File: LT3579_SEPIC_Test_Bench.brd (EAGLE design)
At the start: 74 x 58 mm, 160 parts

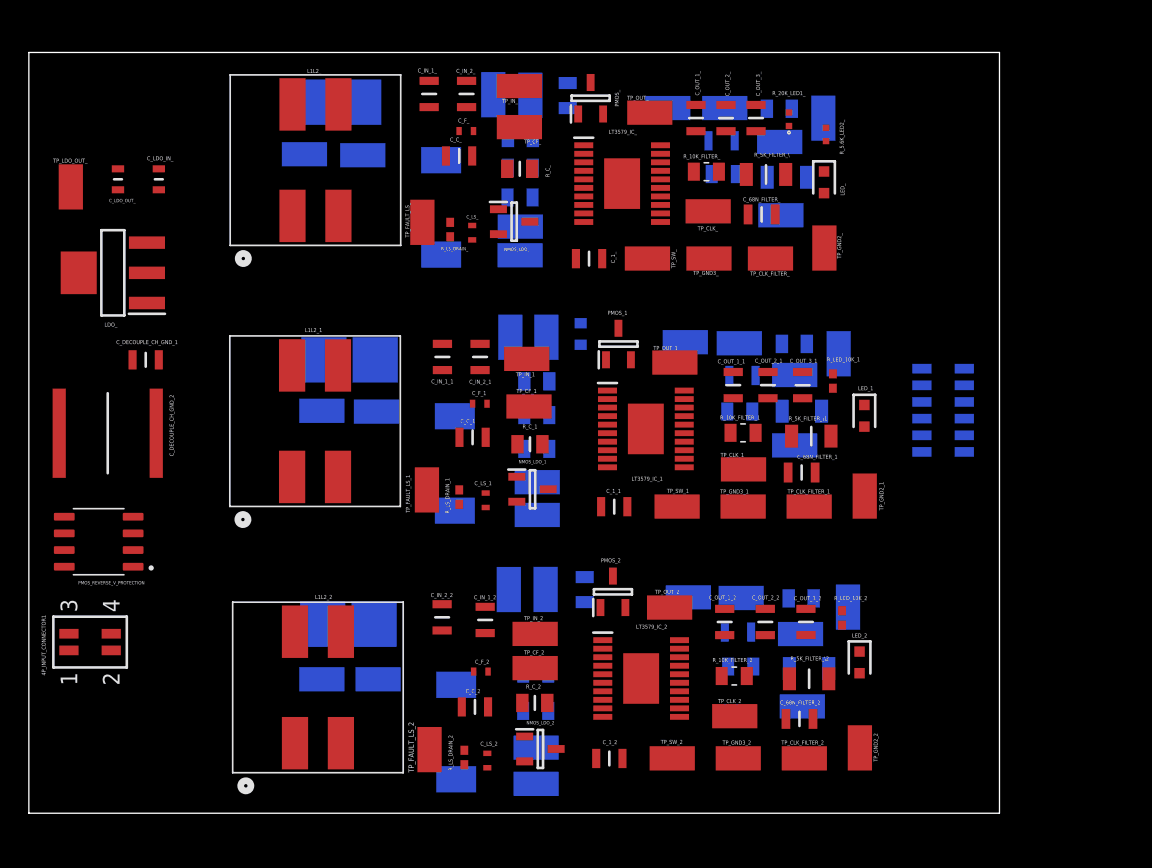
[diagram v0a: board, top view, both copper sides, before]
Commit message: modiefied baord layout
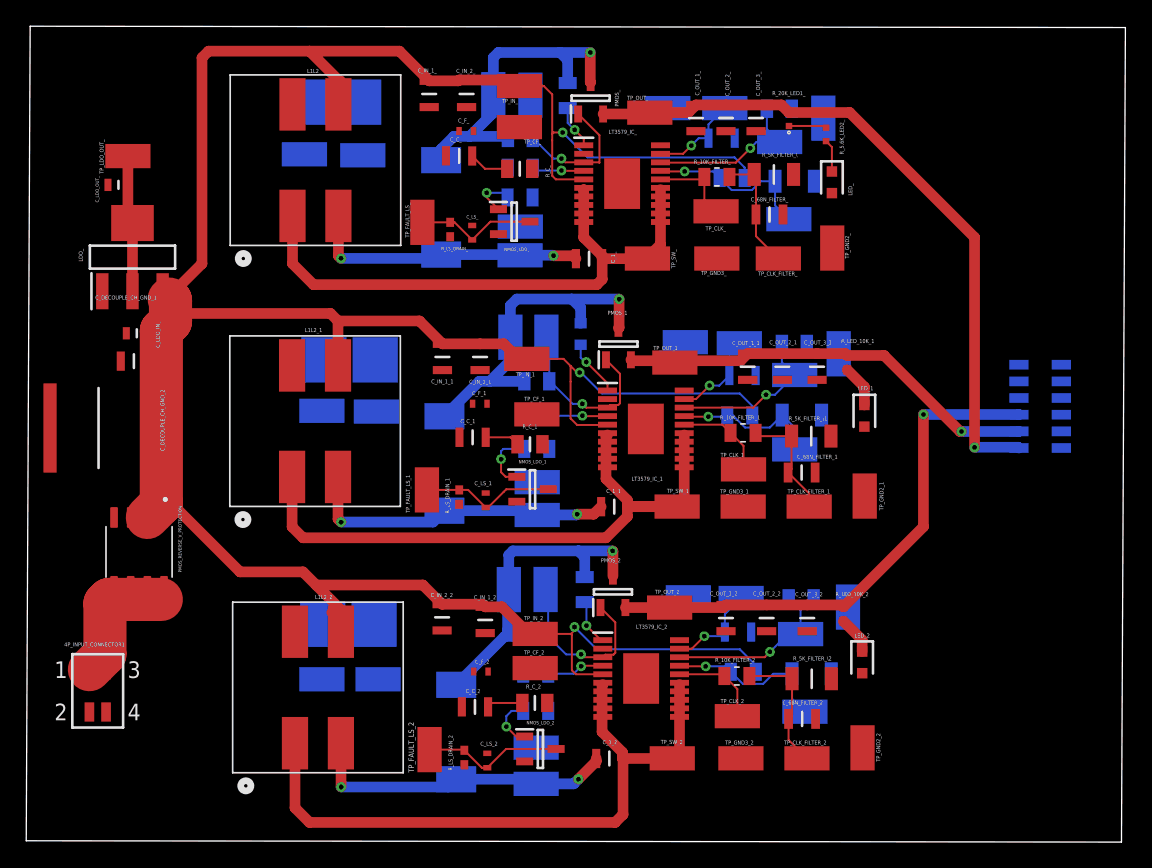
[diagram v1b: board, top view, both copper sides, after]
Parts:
- moved C_LDO_IN_ 11.9 mm to (8.23, 36.6), turned to 180 degrees
- moved 12P_OUTPUT_CONNECTOR1 7.41 mm to (77.1, 31.0)
- moved TP_LDO_OUT_ 4.94 mm to (7.55, 50.1), turned to 180 degrees
- moved 4P_INPUT_CONNECTOR1 3.76 mm to (5.25, 9.33), turned to 0 degrees
- moved PMOS_REVERSE_V_PROTECTION 3.17 mm to (8.40, 19.9), turned to 270 degrees
- moved LDO_ 1.92 mm to (7.90, 42.4), turned to 90 degrees
- moved C_OUT_2_1 1.78 mm to (57.4, 34.0)
- moved C_OUT_3_1 1.78 mm to (60.1, 34.0)
- moved R_LED_10K_1 1.78 mm to (62.4, 34.4)
- moved C_OUT_1_1 1.78 mm to (54.8, 34.0)
- moved C_DECOUPLE_CH_GND_1 0.91 mm to (8.01, 34.5)
- moved R_10K_FILTER_ 0.89 mm to (52.5, 48.5)
- moved TP_CF_1 0.85 mm to (38.7, 30.4)
- moved C_DECOUPLE_CH_GND_2 0.81 mm to (5.31, 29.4)
- moved D1_1 0.80 mm to (31.7, 26.7)
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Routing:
- net VIN: track 0.00 -> 212.9 mm, vias 0 -> 3
- net VOUT_: track 0.00 -> 52.2 mm, vias 0 -> 1
- net SW1-2_2: track 0.00 -> 50.9 mm
- net SW1-2_1: track 0.00 -> 49.5 mm
- net SW1-2_: track 0.00 -> 44.1 mm
- net VOUT_2: track 0.00 -> 41.2 mm, vias 0 -> 1
- net VOUT_1: track 0.00 -> 32.3 mm, vias 0 -> 1
- net N$3: track 0.00 -> 26.5 mm, vias 0 -> 1
- net N$7: track 0.00 -> 25.3 mm, vias 0 -> 1
- net N$13: track 0.00 -> 24.6 mm, vias 0 -> 1
- net N$1: track 0.00 -> 24.1 mm, vias 0 -> 2
- net N$5: track 0.00 -> 24.1 mm, vias 0 -> 2
- net N$9: track 0.00 -> 21.5 mm, vias 0 -> 2
- net GATE_: track 0.00 -> 13.6 mm, vias 0 -> 1
- net GATE_2: track 0.00 -> 13.5 mm, vias 0 -> 1
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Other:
- board size 74 x 58 mm -> 83.8 x 62.2 mm
